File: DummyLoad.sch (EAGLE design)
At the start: 34 parts, among them IC1 LM358, J1 BINDING-POST, J10 PINHD-1X1, J2 BINDING-POST, J3 PINHD-1X1, J4 PINHD-1X1, J5 PINHD-1X1, J6 POWERJACK-OFFBRD, J7 PINHD-1X1, J8 PINHD-1X1, J9 PINHD-1X1, Q1 NTE2390, SW1 SWITCH-SPDT-OFFBRD, SW2 SWITCH-SPDT-OFFBRD, U1 LP2950

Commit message: Clean up layout
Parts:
- C4: device SaintGimp:CAP-POL-2.5-5 -> SaintGimp:CAP-POL-2.5-6
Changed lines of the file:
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@@
 <part name="J6" library="SaintGimp" deviceset="POWERJACK" device="-OFFBRD"/>
 <part name="U1" library="SaintGimp" deviceset="LP2950" device=""/>
-<part name="C4" library="SaintGimp" deviceset="CAP-POL" device="-2.5-5" value="100uF"/>
-<part name="C5" library="SaintGimp" deviceset="CAP-POL" device="-2.5-5" value="2.2uF"/>
+<part name="C4" library="SaintGimp" deviceset="CAP-POL-*" device="2.5-6" value="100uF"/>
+<part name="C5" library="SaintGimp" deviceset="CAP-POL-*" device="2.5-5" value="2.2uF"/>
 <part name="PM1" library="SaintGimp" deviceset="PANEL-METER" device="-OFFBRD"/>
 <part name="J7" library="SaintGimp" deviceset="PINHD-1X1" device=""/>
@@
 <instance part="RV2" gate="G$1" x="12.7" y="33.02"/>
 <instance part="R4" gate="G$1" x="12.7" y="45.72" rot="R90"/>
-<instance part="J3" gate="G$1" x="78.74" y="60.96" smashed="yes" rot="R180">
+<instance part="J3" gate="1" x="78.74" y="60.96" smashed="yes" rot="R180">
 <attribute name="NAME" x="74.93" y="62.611" size="1.778" layer="95"/>
 </instance>
-<instance part="J4" gate="G$1" x="76.2" y="45.72" smashed="yes" rot="R180">
+<instance part="J4" gate="1" x="76.2" y="45.72" smashed="yes" rot="R180">
 <attribute name="NAME" x="72.39" y="47.371" size="1.778" layer="95"/>
 </instance>
 <instance part="GND4" gate="1" x="68.58" y="30.48" rot="R270"/>
-<instance part="J5" gate="G$1" x="78.74" y="30.48" smashed="yes" rot="R180">
+<instance part="J5" gate="1" x="78.74" y="30.48" smashed="yes" rot="R180">
 <attribute name="NAME" x="74.93" y="32.131" size="1.778" layer="95"/>
 </instance>
@@
 <instance part="C5" gate="G$1" x="27.94" y="81.28"/>
 <instance part="PM1" gate="G$1" x="121.92" y="91.44"/>
-<instance part="J7" gate="G$1" x="78.74" y="93.98" smashed="yes" rot="R180">
+<instance part="J7" gate="1" x="78.74" y="93.98" smashed="yes" rot="R180">
 <attribute name="NAME" x="74.93" y="95.631" size="1.778" layer="95"/>
 </instance>
 <instance part="GND9" gate="1" x="68.58" y="78.74" rot="R270"/>
-<instance part="J8" gate="G$1" x="78.74" y="78.74" smashed="yes" rot="R180">
+<instance part="J8" gate="1" x="78.74" y="78.74" smashed="yes" rot="R180">
 <attribute name="NAME" x="74.93" y="80.391" size="1.778" layer="95"/>
 </instance>
 <instance part="GND10" gate="1" x="68.58" y="86.36" rot="R270"/>
-<instance part="J9" gate="G$1" x="78.74" y="86.36" smashed="yes" rot="R180">
+<instance part="J9" gate="1" x="78.74" y="86.36" smashed="yes" rot="R180">
 <attribute name="NAME" x="74.93" y="88.011" size="1.778" layer="95"/>
 </instance>
@@
 <instance part="RV3" gate="G$1" x="25.4" y="96.52" rot="R270"/>
 <instance part="GND1" gate="1" x="15.24" y="96.52" rot="R270"/>
-<instance part="J10" gate="G$1" x="76.2" y="106.68" smashed="yes" rot="R180">
+<instance part="J10" gate="1" x="76.2" y="106.68" smashed="yes" rot="R180">
 <attribute name="NAME" x="72.39" y="108.331" size="1.778" layer="95"/>
 </instance>
@@
 <segment>
 <pinref part="GND4" gate="1" pin="GND"/>
-<pinref part="J5" gate="G$1" pin="KL"/>
+<pinref part="J5" gate="1" pin="KL"/>
 <wire x1="71.12" y1="30.48" x2="73.66" y2="30.48" width="0.1524" layer="91"/>
 <label x="78.74" y="30.48" size="1.778" layer="95" xref="yes"/>
@@
 <segment>
 <pinref part="GND9" gate="1" pin="GND"/>
-<pinref part="J8" gate="G$1" pin="KL"/>
+<pinref part="J8" gate="1" pin="KL"/>
 <wire x1="71.12" y1="78.74" x2="73.66" y2="78.74" width="0.1524" layer="91"/>
 <label x="78.74" y="78.74" size="1.778" layer="95" xref="yes"/>
@@
 <segment>
 <pinref part="GND10" gate="1" pin="GND"/>
-<pinref part="J9" gate="G$1" pin="KL"/>
+<pinref part="J9" gate="1" pin="KL"/>
 <wire x1="71.12" y1="86.36" x2="73.66" y2="86.36" width="0.1524" layer="91"/>
 <label x="78.74" y="86.36" size="1.778" layer="95" xref="yes"/>
@@
 <segment>
 <pinref part="R1" gate="G$1" pin="1"/>
-<pinref part="J3" gate="G$1" pin="KL"/>
+<pinref part="J3" gate="1" pin="KL"/>
 <label x="78.74" y="60.96" size="1.778" layer="95" xref="yes"/>
 <wire x1="73.66" y1="60.96" x2="68.58" y2="60.96" width="0.1524" layer="91"/>
@@
 <junction x="27.94" y="83.82"/>
 <label x="78.74" y="93.98" size="1.778" layer="95" xref="yes"/>
-<pinref part="J7" gate="G$1" pin="KL"/>
+<pinref part="J7" gate="1" pin="KL"/>
 <wire x1="73.66" y1="93.98" x2="45.72" y2="93.98" width="0.1524" layer="91"/>
 <wire x1="45.72" y1="93.98" x2="45.72" y2="83.82" width="0.1524" layer="91"/>
@@
 <segment>
 <pinref part="R2" gate="G$1" pin="2"/>
-<pinref part="J4" gate="G$1" pin="KL"/>
+<pinref part="J4" gate="1" pin="KL"/>
 <wire x1="71.12" y1="45.72" x2="68.58" y2="45.72" width="0.1524" layer="91"/>
 <label x="76.2" y="45.72" size="1.778" layer="95" xref="yes"/>
@@
 <pinref part="IC1" gate="G2" pin="OUT"/>
 <pinref part="R6" gate="G$1" pin="2"/>
-<pinref part="J10" gate="G$1" pin="KL"/>
+<pinref part="J10" gate="1" pin="KL"/>
 <junction x="71.12" y="106.68"/>
 <label x="76.2" y="106.68" size="1.778" layer="95" xref="yes"/>

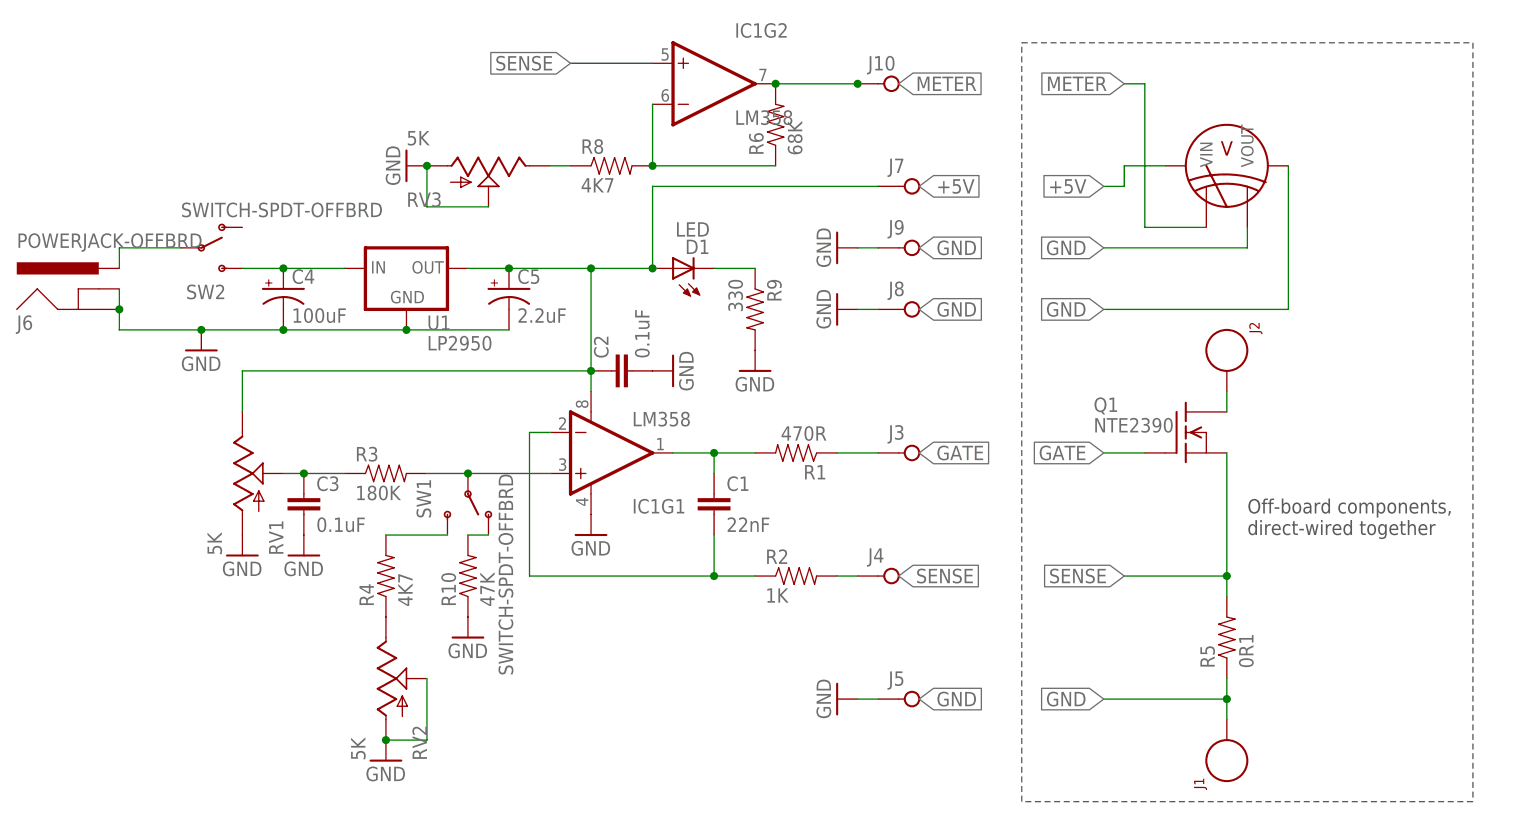
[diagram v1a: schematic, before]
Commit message: Design updates
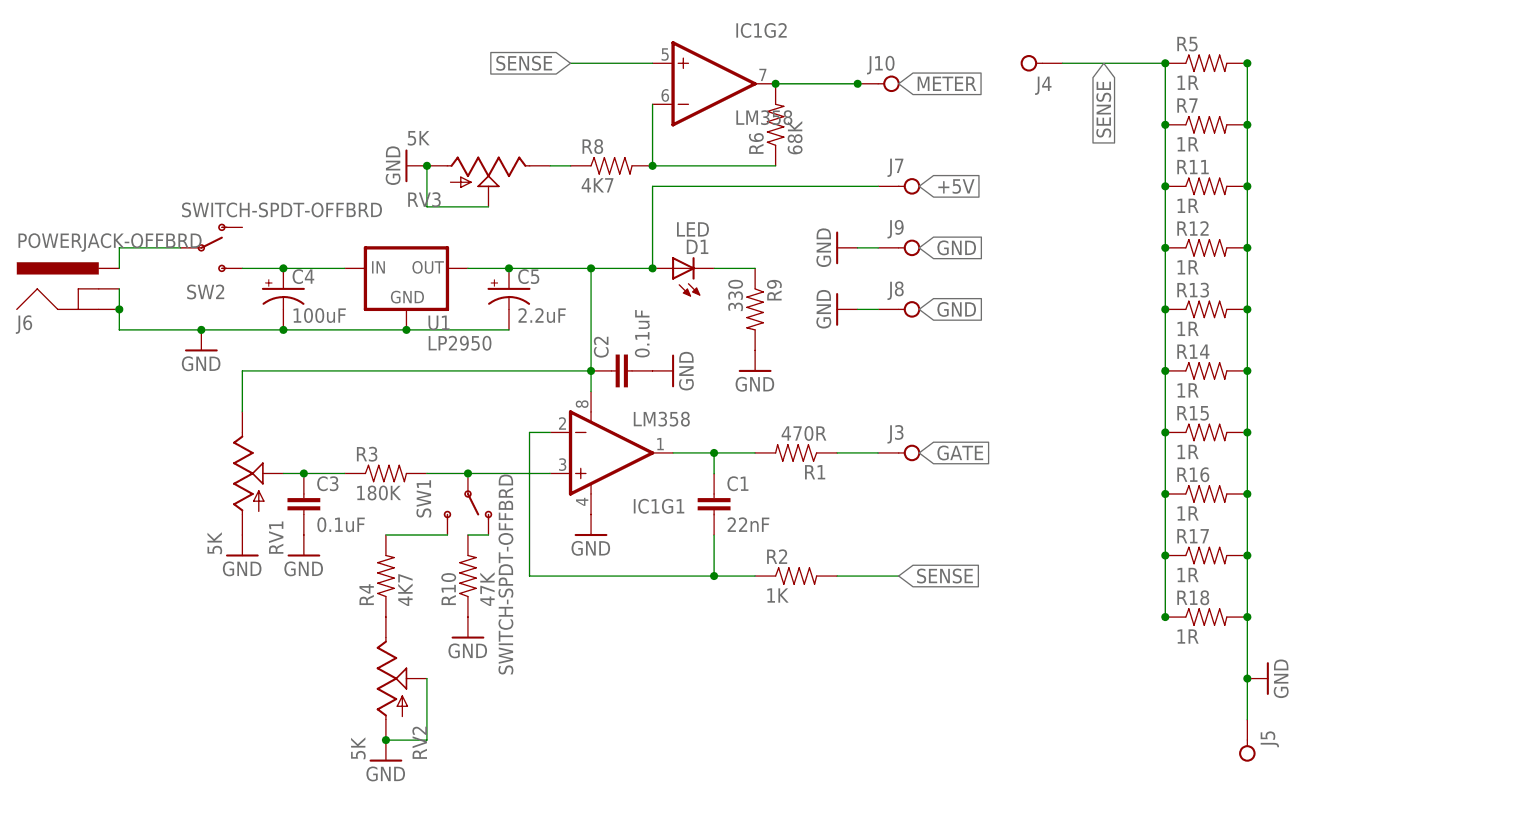
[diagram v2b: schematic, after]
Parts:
- removed J1, J2: BINDING-POST, SaintGimp:BINDING-POST
- removed PM1: PANEL-METER-OFFBRD, SaintGimp:PANEL-METER-OFFBRD
- removed Q1: NTE2390, SaintGimp:NTE2390
- added R11, R12, R13, R14, R15, R16, R17, R18, R7: 1R, SaintGimp:RESISTOR-7.5MM
- R5: value 0R1 -> 1R
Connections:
- removed net N$7: J2.1, Q1.DRN
- net +5V: no longer PM1.+5V
- net GATE: no longer Q1.GATE
- net GND: now also R11.2, R12.2, R13.2, R14.2, R15.2, R16.2, R17.2, R18.2, R5.2, R7.2; no longer J1.1, PM1.GND, PM1.VOUT, R5.1
- net METER: no longer PM1.VIN
- net SENSE: now also R11.1, R12.1, R13.1, R14.1, R15.1, R16.1, R17.1, R18.1, R5.1, R7.1; no longer Q1.SRC, R5.2
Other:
- note removed: "Off-board components, direct-wired together"
- moved on the sheet: J4, J5, R5
